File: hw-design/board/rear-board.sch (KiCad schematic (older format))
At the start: 12 parts, among them J1 CC_MAIN, J2 CC_NEXT, P6 CONN_01X12, P7 USB_OTG, P8 CONN_01X12, Q6 IRFML8244TRPBF

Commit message: set RJ45 footprint
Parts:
- J1, J2: footprint (none) -> local-footprints:54602-908LF
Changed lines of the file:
@@
 F 0 "J1" V 2900 1850 50  0000 L CNN
 F 1 "CC_MAIN" H 2450 2350 50  0000 C CNN
-F 2 "" H 2450 1850 50  0000 C CNN
+F 2 "local-footprints:54602-908LF" H 2450 1850 50  0001 C CNN
 F 3 "" H 2450 1850 50  0000 C CNN
 	1    2450 1850
@@
 F 0 "J2" V 2900 3250 50  0000 L CNN
 F 1 "CC_NEXT" H 2450 3750 50  0000 C CNN
-F 2 "" H 2450 3250 50  0000 C CNN
+F 2 "local-footprints:54602-908LF" H 2450 3250 50  0001 C CNN
 F 3 "" H 2450 3250 50  0000 C CNN
 	1    2450 3250

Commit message: changing footprint of rear board header
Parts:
- P6: footprint Pin_Headers:Pin_Header_Straight_1x12 -> Pin_Headers:Pin_Header_Angled_1x12
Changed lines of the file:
@@
 F 0 "P6" H 8550 2650 50  0000 C CNN
 F 1 "CONN_01X12" V 8650 2000 50  0000 C CNN
-F 2 "Pin_Headers:Pin_Header_Straight_1x12" H 8550 2000 60  0001 C CNN
+F 2 "Pin_Headers:Pin_Header_Angled_1x12" H 8550 2000 60  0001 C CNN
 F 3 "" H 8550 2000 60  0000 C CNN
 	1    8550 2000

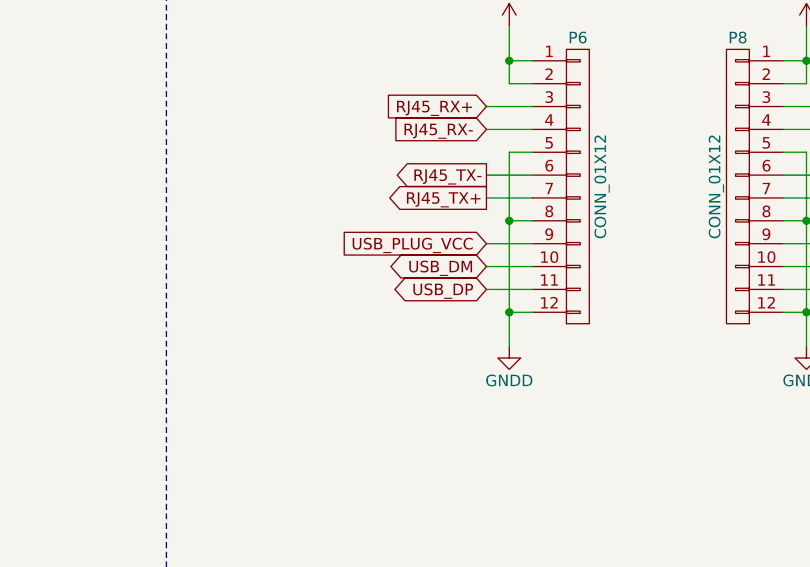
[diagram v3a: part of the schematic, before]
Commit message: fix usb resistors
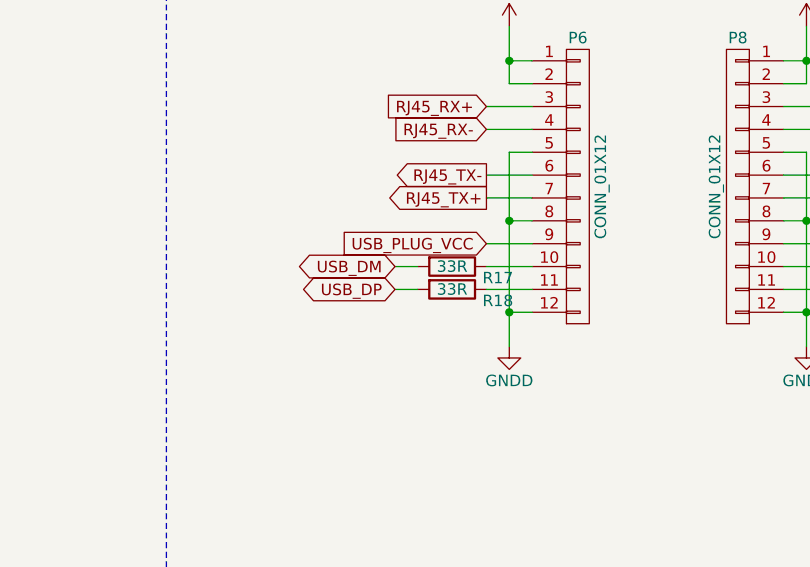
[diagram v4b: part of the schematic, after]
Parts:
- added R17, R18: 33R, Resistors_SMD:R_0603, symbol R
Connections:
- net USB_DM: now also R17.2; no longer P6.10 (P10)
- net USB_DP: now also R18.2; no longer P6.11 (P11)
- new net: P6.10 (P10), R17.1
- new net: P6.11 (P11), R18.1
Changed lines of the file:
@@
 	-1   0    0    -1
 $EndComp
-Text GLabel 8150 2350 0    50   BiDi ~ 0
+Text GLabel 7750 2350 0    50   BiDi ~ 0
 USB_DM
-Text GLabel 8150 2450 0    50   BiDi ~ 0
+Text GLabel 7750 2450 0    50   BiDi ~ 0
 USB_DP
 Text GLabel 9650 2350 2    50   BiDi ~ 0
@@
 	1    0    0    -1
 $EndComp
-Wire Wire Line
-	2900 1500 3000 1500
-Wire Wire Line
-	2900 1600 3000 1600
-Wire Wire Line
-	3000 1700 2900 1700
-Wire Wire Line
-	3000 2000 2900 2000
-Wire Wire Line
-	2900 2100 3000 2100
-Wire Wire Line
-	3000 2100 3000 2300
-Wire Wire Line
-	2900 2200 3000 2200
-Wire Wire Line
-	4150 3950 4150 4050
-Wire Wire Line
-	3900 3500 4500 3500
-Wire Wire Line
-	4150 3350 4150 3650
-Wire Wire Line
-	4150 3050 4150 2950
-Connection ~ 3000 2200
-Connection ~ 4150 3500
-Wire Wire Line
-	8150 1650 8350 1650
-Wire Wire Line
-	8350 1750 8150 1750
-Wire Wire Line
-	8150 2050 8350 2050
-Wire Wire Line
-	8350 1950 8150 1950
-Wire Wire Line
-	8150 2250 8350 2250
-Wire Wire Line
-	8150 2350 8350 2350
-Wire Wire Line
-	8350 2450 8150 2450
-Wire Wire Line
-	8450 5050 8450 4950
-Wire Wire Line
-	8250 4950 8550 4950
-Wire Wire Line
-	8250 4950 8250 5050
-Wire Wire Line
-	8250 5350 8250 5450
-Wire Wire Line
-	8250 5450 8750 5450
-Wire Wire Line
-	8750 5450 8750 5350
-Wire Wire Line
-	8450 5350 8450 5550
-Connection ~ 8450 4950
-Connection ~ 8450 5450
-Wire Wire Line
-	9150 5350 9150 5500
-Wire Wire Line
-	9150 5500 9250 5500
-Wire Wire Line
-	9250 5600 9050 5600
-Wire Wire Line
-	9050 5600 9050 5350
-Wire Wire Line
-	8950 5350 8950 5700
-Wire Wire Line
-	8950 5700 9250 5700
-Wire Wire Line
-	3600 6200 3600 6100
-Wire Wire Line
-	3700 5550 3600 5550
-Wire Wire Line
-	3600 5550 3600 5700
-Wire Wire Line
-	3700 6650 3600 6650
-Wire Wire Line
-	3600 6650 3600 6500
-Wire Wire Line
-	3100 5900 3300 5900
-Wire Notes Line
-	6750 700  6750 7450
-Wire Notes Line
-	7200 3900 10400 3900
-Wire Wire Line
-	9450 1650 9650 1650
-Wire Wire Line
-	9650 1750 9450 1750
-Wire Wire Line
-	9450 2050 9650 2050
-Wire Wire Line
-	9650 1950 9450 1950
-Wire Wire Line
-	9650 2350 9450 2350
-Wire Wire Line
-	9450 2450 9650 2450
-Wire Wire Line
-	9650 2250 9450 2250
 $Comp
 L RJ45 J1
@@
 	0    -1   1    0
 $EndComp
-Wire Wire Line
-	2900 1900 3550 1900
-Wire Wire Line
-	3550 1900 3550 1800
-Wire Wire Line
-	2900 1800 3000 1800
-Wire Wire Line
-	3000 1800 3000 1900
-Connection ~ 3000 1900
 $Comp
 L GNDD #PWR26
@@
 	1    0    0    -1
 $EndComp
-Wire Wire Line
-	2900 2900 3000 2900
-Wire Wire Line
-	2900 3000 3000 3000
-Wire Wire Line
-	3000 3100 2900 3100
-Wire Wire Line
-	3000 3400 2900 3400
 $Comp
 L RJ45 J2
@@
 	0    -1   1    0
 $EndComp
-Wire Wire Line
-	2900 3300 3550 3300
-Wire Wire Line
-	3550 3300 3550 3200
-Wire Wire Line
-	2900 3200 3000 3200
-Wire Wire Line
-	3000 3200 3000 3300
-Connection ~ 3000 3300
 NoConn ~ 2100 2400
 NoConn ~ 2100 3800
-Wire Wire Line
-	2900 3600 3000 3600
-Wire Wire Line
-	3000 3600 3000 3700
-Wire Wire Line
-	2900 3500 3600 3500
 $Comp
 L +12V #PWR62
@@
 	1    0    0    -1
 $EndComp
-Wire Wire Line
-	8250 1300 8250 1550
 $Comp
 L +12V #PWR76
@@
 	1    0    0    -1
 $EndComp
+$Comp
+L R R17
+U 1 1 576041F9
+P 8000 2350
+F 0 "R17" V 8050 2550 50  0000 C CNN
+F 1 "33R" V 8000 2350 50  0000 C CNN
+F 2 "Resistors_SMD:R_0603" V 7930 2350 30  0001 C CNN
+F 3 "" H 8000 2350 30  0000 C CNN
+F 4 "MCR03ERTF33R0" H 4000 -4850 50  0001 C CNN "MPN"
+	1    8000 2350
+	0    1    1    0
+$EndComp
+$Comp
+L R R18
+U 1 1 57604201
+P 8000 2450
+F 0 "R18" V 8050 2650 50  0000 C CNN
+F 1 "33R" V 8000 2450 50  0000 C CNN
+F 2 "Resistors_SMD:R_0603" V 7930 2450 30  0001 C CNN
+F 3 "" H 8000 2450 30  0000 C CNN
+F 4 "MCR03ERTF33R0" H 4000 -4900 50  0001 C CNN "MPN"
+	1    8000 2450
+	0    1    1    0
+$EndComp
+Wire Wire Line
+	2900 1500 3000 1500
+Wire Wire Line
+	2900 1600 3000 1600
+Wire Wire Line
+	3000 1700 2900 1700
+Wire Wire Line
+	3000 2000 2900 2000
+Wire Wire Line
+	2900 2100 3000 2100
+Wire Wire Line
+	3000 2100 3000 2300
+Wire Wire Line
+	2900 2200 3000 2200
+Wire Wire Line
+	4150 3950 4150 4050
+Wire Wire Line
+	3900 3500 4500 3500
+Wire Wire Line
+	4150 3350 4150 3650
+Wire Wire Line
+	4150 3050 4150 2950
+Connection ~ 3000 2200
+Connection ~ 4150 3500
+Wire Wire Line
+	8150 1650 8350 1650
+Wire Wire Line
+	8350 1750 8150 1750
+Wire Wire Line
+	8150 2050 8350 2050
+Wire Wire Line
+	8350 1950 8150 1950
+Wire Wire Line
+	8150 2250 8350 2250
+Wire Wire Line
+	8150 2350 8350 2350
+Wire Wire Line
+	8350 2450 8150 2450
+Wire Wire Line
+	8450 5050 8450 4950
+Wire Wire Line
+	8250 4950 8550 4950
+Wire Wire Line
+	8250 4950 8250 5050
+Wire Wire Line
+	8250 5350 8250 5450
+Wire Wire Line
+	8250 5450 8750 5450
+Wire Wire Line
+	8750 5450 8750 5350
+Wire Wire Line
+	8450 5350 8450 5550
+Connection ~ 8450 4950
+Connection ~ 8450 5450
+Wire Wire Line
+	9150 5350 9150 5500
+Wire Wire Line
+	9150 5500 9250 5500
+Wire Wire Line
+	9250 5600 9050 5600
+Wire Wire Line
+	9050 5600 9050 5350
+Wire Wire Line
+	8950 5350 8950 5700
+Wire Wire Line
+	8950 5700 9250 5700
+Wire Wire Line
+	3600 6200 3600 6100
+Wire Wire Line
+	3700 5550 3600 5550
+Wire Wire Line
+	3600 5550 3600 5700
+Wire Wire Line
+	3700 6650 3600 6650
+Wire Wire Line
+	3600 6650 3600 6500
+Wire Wire Line
+	3100 5900 3300 5900
+Wire Notes Line
+	6750 700  6750 7450
+Wire Notes Line
+	7200 3900 10400 3900
+Wire Wire Line
+	9450 1650 9650 1650
+Wire Wire Line
+	9650 1750 9450 1750
+Wire Wire Line
+	9450 2050 9650 2050
+Wire Wire Line
+	9650 1950 9450 1950
+Wire Wire Line
+	9650 2350 9450 2350
+Wire Wire Line
+	9450 2450 9650 2450
+Wire Wire Line
+	9650 2250 9450 2250
+Wire Wire Line
+	2900 1900 3550 1900
+Wire Wire Line
+	3550 1900 3550 1800
+Wire Wire Line
+	2900 1800 3000 1800
+Wire Wire Line
+	3000 1800 3000 1900
+Connection ~ 3000 1900
+Wire Wire Line
+	2900 2900 3000 2900
+Wire Wire Line
+	2900 3000 3000 3000
+Wire Wire Line
+	3000 3100 2900 3100
+Wire Wire Line
+	3000 3400 2900 3400
+Wire Wire Line
+	2900 3300 3550 3300
+Wire Wire Line
+	3550 3300 3550 3200
+Wire Wire Line
+	2900 3200 3000 3200
+Wire Wire Line
+	3000 3200 3000 3300
+Connection ~ 3000 3300
+Wire Wire Line
+	2900 3600 3000 3600
+Wire Wire Line
+	3000 3600 3000 3700
+Wire Wire Line
+	2900 3500 3600 3500
+Wire Wire Line
+	8250 1300 8250 1550
 Wire Wire Line
 	9550 1300 9550 1550
@@
 	9450 2150 9550 2150
 Connection ~ 9550 2150
+Wire Wire Line
+	7750 2350 7850 2350
+Wire Wire Line
+	7850 2450 7750 2450
 $EndSCHEMATC
